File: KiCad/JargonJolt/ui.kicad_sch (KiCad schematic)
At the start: 0 parts

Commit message: worked on pinout
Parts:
- added C1, C2, C3: 0.1uF, symbol Device:C
- added R1, R3, R5: 1k, symbol Device:R
- added R2, R4, R6: 10k, symbol Device:R
- added SW1, SW2, SW3: SW_Push, symbol Switch:SW_Push
- added U1, U2, U3: 40106, symbol 4xxx:40106
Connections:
- new net: R3.2, R4.2, SW2.2
- new net: C1.1, R1.1, U1.1
- new net: R5.2, R6.2, SW3.2
- new net: C3.1, R5.1, U3.1
- new net: R1.2, R2.2, SW1.2
- new net: C2.1, R3.1, U2.1
- new net +3.3V: R2.1, R4.1, R6.1
- new net BUTTON1: U1.2
- new net BUTTON2: U2.2
- new net BUTTON3: U3.2
- new net GND: C1.2, C2.2, C3.2, SW1.1, SW2.1, SW3.1

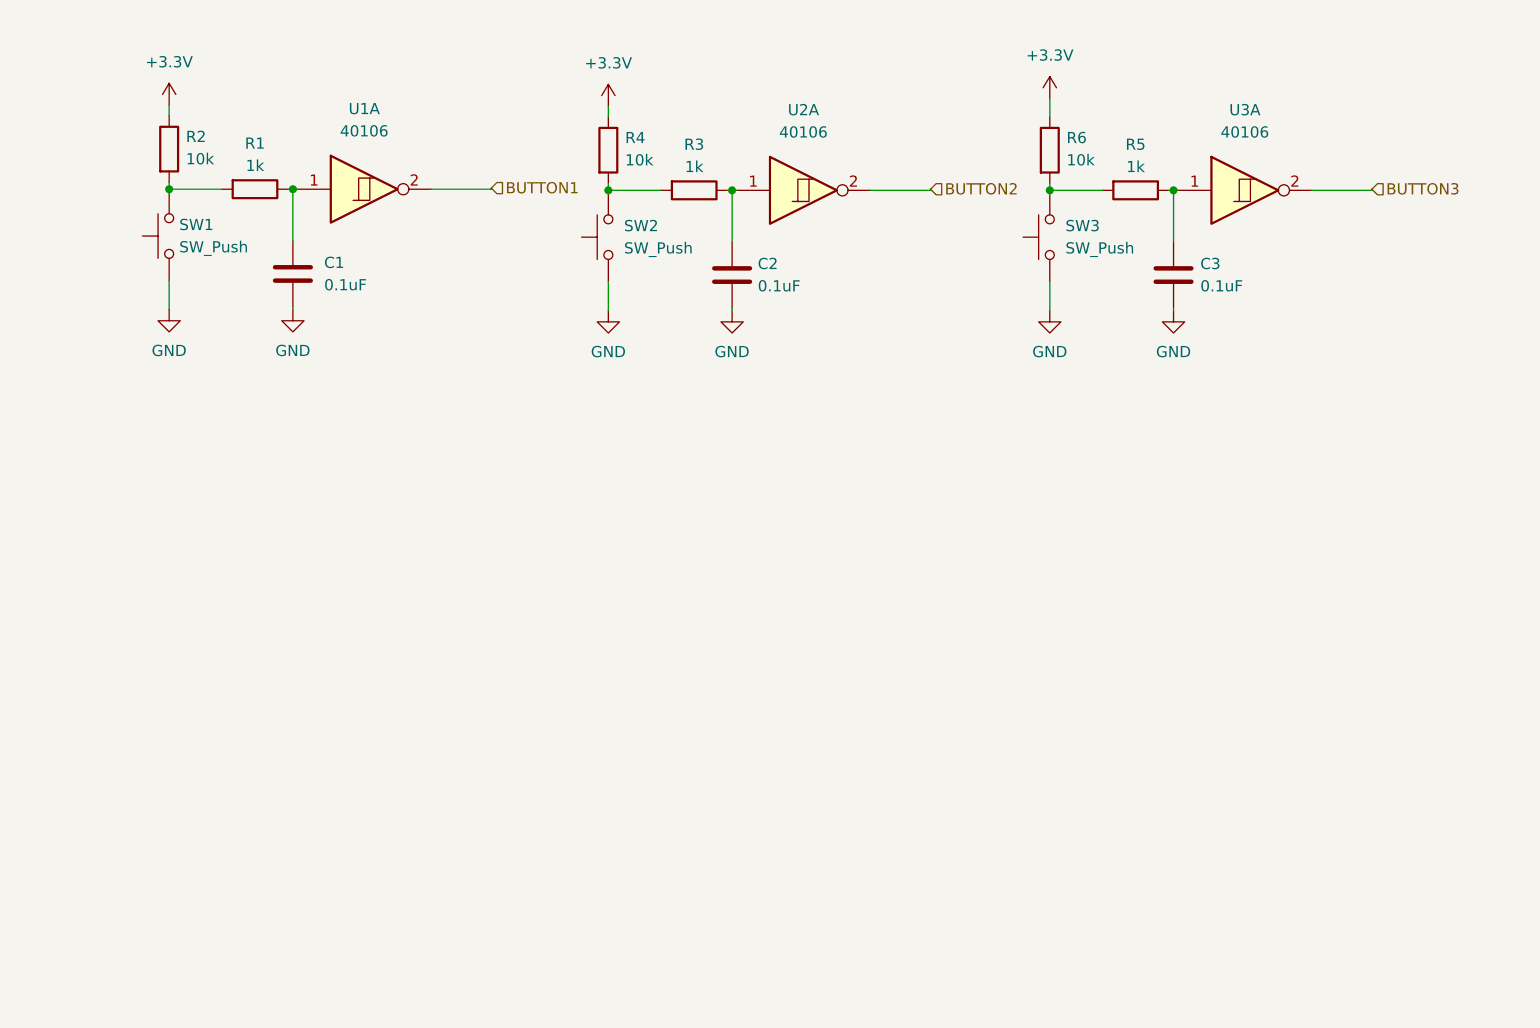
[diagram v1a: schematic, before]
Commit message: worked on schematic
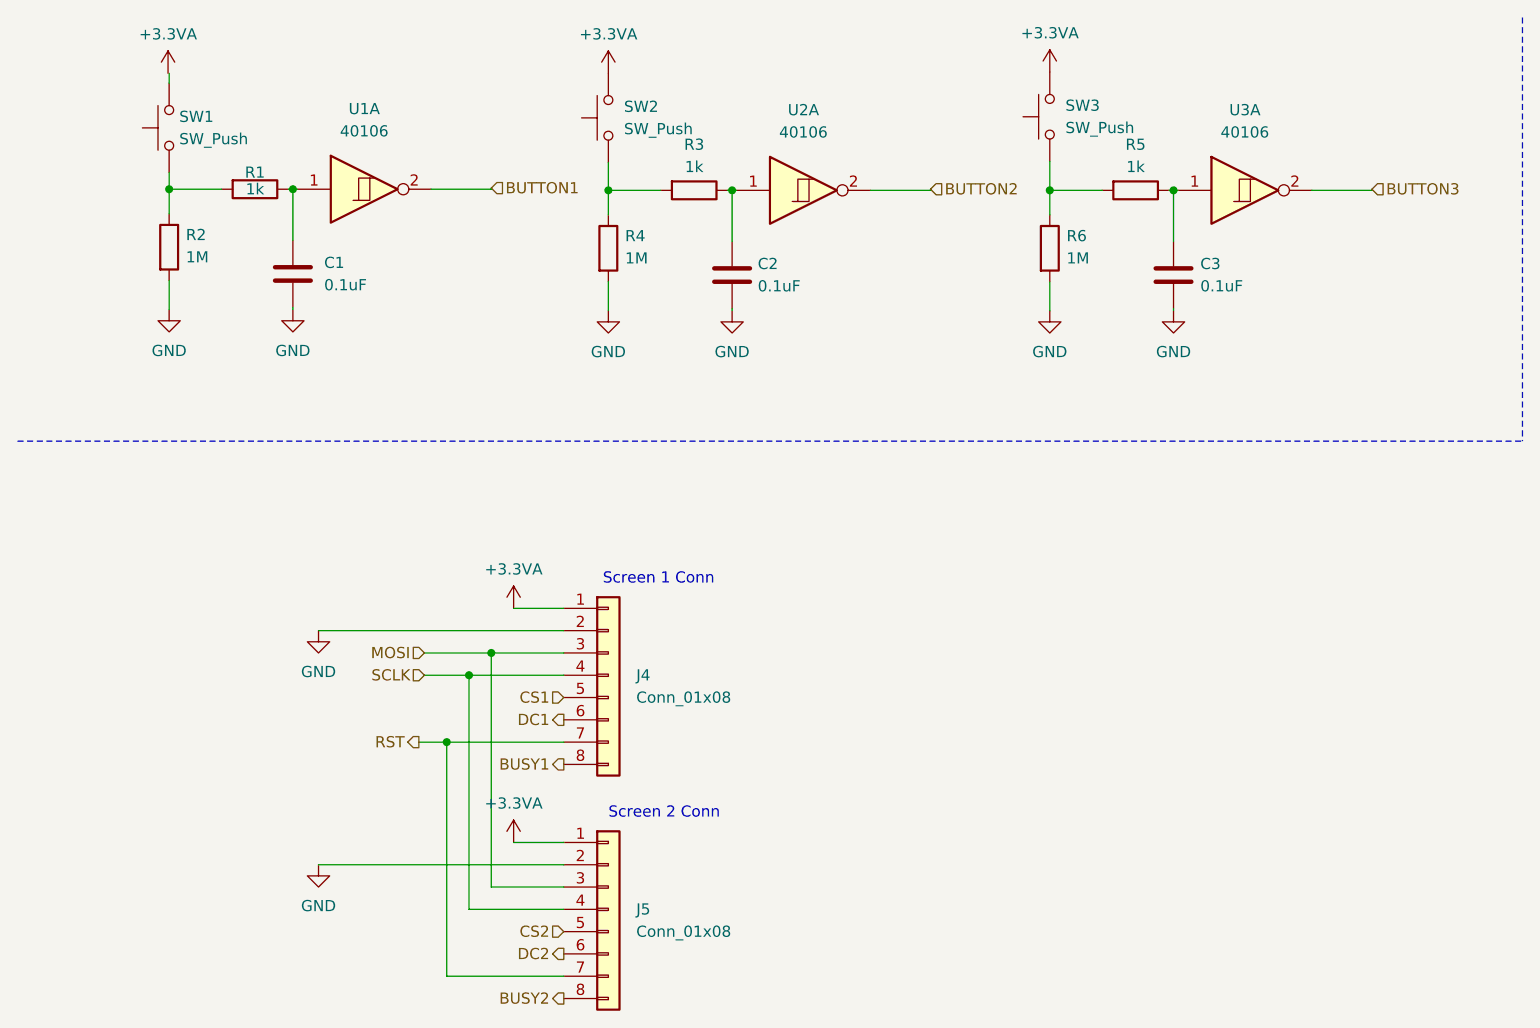
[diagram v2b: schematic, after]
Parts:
- added J4, J5: Conn_01x08, symbol Connector_Generic:Conn_01x08
- R2, R4, R6: value 10k -> 1M
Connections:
- net GND: now also R2.2, R4.2, R6.2, J4.2 (Pin_2), J5.2 (Pin_2); no longer SW1.1, SW2.1, SW3.1
- removed net +3.3V: R2.1, R4.1, R6.1
- new net: R3.2, R4.1, SW2.1
- new net: R5.2, R6.1, SW3.1
- new net: R1.2, R2.1, SW1.1
- new net +3.3VA: J4.1 (Pin_1), J5.1 (Pin_1), SW2.2, SW3.2
- new net BUSY1: J4.8 (Pin_8)
- new net BUSY2: J5.8 (Pin_8)
- new net CS1: J4.5 (Pin_5)
- new net CS2: J5.5 (Pin_5)
- new net DC1: J4.6 (Pin_6)
- new net DC2: J5.6 (Pin_6)
- new net MOSI: J4.3 (Pin_3), J5.3 (Pin_3)
- new net RST: J4.7 (Pin_7), J5.7 (Pin_7)
- new net SCLK: J4.4 (Pin_4), J5.4 (Pin_4)
- now unconnected: SW1.2
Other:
- note added: "Screen 1 Conn"
- note added: "Screen 2 Conn"
- moved on the sheet: R2, R4, R6, SW1, SW2, SW3
